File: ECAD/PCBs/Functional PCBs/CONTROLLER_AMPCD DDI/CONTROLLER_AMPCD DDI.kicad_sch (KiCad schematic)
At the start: 49 parts, among them IC1 THVD1410DR, IC2 TPS563300DRLR, J1 BUS IN, J2 BUS OUT, J3 DDI/AMPCD, J4 BRT/CRS, J5 CONT/HDG, J6 DDI ROT, J7 AMPCD ROT, J8 EWI SW, Q1 AO3400A, Q2 IRLML6402TRPBF

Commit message: Updating Symbols to new/corrected library entries
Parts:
- C2: symbol Device:C -> OH_Symbols:Capacitor_0603_10uF
- C3: symbol Device:C -> OH_Symbols:Capacitor_0402_0.1uF
- D2: LCSC (none) -> C404012
- IC1: LCSC (none) -> C2671345
- Q1: LCSC (none) -> C20917; Manufacture PN (none) -> AO3400A
- R1: symbol Device:R -> OH_Symbols:Resistor_0603_100Ω; LCSC C25804 -> C22775; PN 0603WAF1002T5E -> 0603WAF1000T5E
- R13: symbol Device:R -> OH_Symbols:Resistor_0402_0Ω; LCSC (none) -> C17168; Manufacture PN (none) -> 0402WGF0000TCE
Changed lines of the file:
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@@
 	)
 	(symbol
-		(lib_id "Device:R")
+		(lib_id "OH_Symbols:Resistor_0603_100Ω")
 		(at 33.02 177.8 270)
 		(mirror x)
@@
 			)
 		)
-		(property "Datasheet" "https://datasheet.lcsc.com/szlcsc/1811062009_UNI-ROYAL-Uniroyal-Elec-0603WAF1002T5E_C25804.pdf"
+		(property "Datasheet" "https://www.lcsc.com/datasheet/C22775.pdf"
 			(at 33.02 177.8 0)
 			(hide yes)
@@
 			)
 		)
-		(property "Description" ""
+		(property "Description" "Resistor,, SMD 0603_1608, 100 Ohm"
 			(at 33.02 177.8 0)
+			(hide yes)
 			(show_name no)
 			(do_not_autoplace no)
@@
 			)
 		)
-		(property "PN" "0603WAF1002T5E"
+		(property "PN" "0603WAF1000T5E"
 			(at 33.02 177.8 90)
 			(hide yes)
@@
 			)
 		)
-		(property "LCSC" "C25804"
+		(property "LCSC" "C22775"
 			(at 33.02 177.8 90)
 			(hide yes)
@@
 			)
 		)
+		(property "LCSC" "C20917"
+			(at 44.45 177.8 0)
+			(hide yes)
+			(show_name no)
+			(do_not_autoplace no)
+			(effects
+				(font
+					(size 1.27 1.27)
+				)
+			)
+		)
+		(property "Manufacture PN" "AO3400A"
+			(at 44.45 177.8 0)
+			(hide yes)
+			(show_name no)
+			(do_not_autoplace no)
+			(effects
+				(font
+					(size 1.27 1.27)
+				)
+			)
+		)
 		(pin "1"
 		)
@@
 			)
 		)
+		(property "LCSC" "C2671345"
+			(at 205.74 123.19 0)
+			(hide yes)
+			(show_name no)
+			(do_not_autoplace no)
+			(effects
+				(font
+					(size 1.27 1.27)
+				)
+			)
+		)
 		(pin "8"
 		)
@@
 	)
 	(symbol
-		(lib_id "Device:C")
+		(lib_id "OH_Symbols:Capacitor_0402_0.1uF")
 		(at 67.31 115.57 180)
 		(unit 1)
@@
 			)
 		)
-		(property "Description" ""
+		(property "Description" "Capacitor, Non-polarized, SMD 0402_1005, 0.1uF"
 			(at 70.231 117.9943 0)
+			(hide yes)
 			(show_name no)
 			(do_not_autoplace no)
@@
 	)
 	(symbol
-		(lib_id "Device:R")
+		(lib_id "OH_Symbols:Resistor_0402_0Ω")
 		(at 106.68 104.14 90)
 		(unit 1)
@@
 			)
 		)
-		(property "Datasheet" ""
+		(property "Datasheet" "https://www.lcsc.com/datasheet/C17168.pdf"
+			(at 106.68 104.14 0)
+			(hide yes)
+			(show_name no)
+			(do_not_autoplace no)
+			(effects
+				(font
+					(size 1.27 1.27)
+				)
+			)
+		)
+		(property "Description" "Resistor,, SMD 0402_1005, 0 Ohm"
+			(at 106.68 104.14 0)
+			(hide yes)
+			(show_name no)
+			(do_not_autoplace no)
+			(effects
+				(font
+					(size 1.27 1.27)
+				)
+			)
+		)
+		(property "LCSC" "C17168"
 			(at 106.68 104.14 0)
 			(hide yes)
@@
 			)
 		)
-		(property "Description" "Resistor"
+		(property "Manufacture PN" "0402WGF0000TCE"
 			(at 106.68 104.14 0)
 			(hide yes)
@@
 	)
 	(symbol
-		(lib_id "Device:C")
+		(lib_id "OH_Symbols:Capacitor_0603_10uF")
 		(at 60.96 115.57 0)
 		(mirror x)
@@
 			)
 		)
-		(property "Description" ""
+		(property "Description" "Capacitor, Non-polarized, SMD 0603_1608, 10uF"
 			(at 58.039 117.9943 0)
+			(hide yes)
 			(show_name no)
 			(do_not_autoplace no)
@@
 			)
 		)
+		(property "LCSC" "C404012"
+			(at 246.38 127 0)
+			(hide yes)
+			(show_name no)
+			(do_not_autoplace no)
+			(effects
+				(font
+					(size 1.27 1.27)
+				)
+			)
+		)

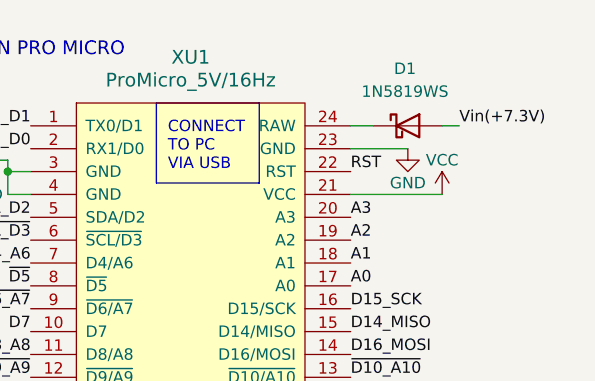
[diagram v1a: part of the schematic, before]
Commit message: Created MCAD and ECAD Release
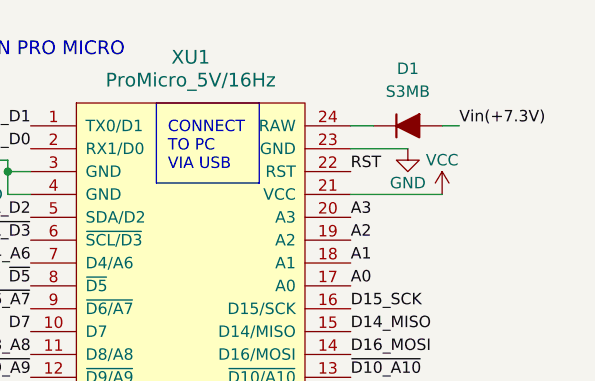
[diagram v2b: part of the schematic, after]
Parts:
- removed D1: 1N5819WS, Diode_SMD:D_SOD-323_HandSoldering, symbol OH_Symbols:1N5819WS
- added D1: S3MB, Diode_SMD:D_SMB, symbol OH_Symbols:D_Filled
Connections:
- net Vin(+7.3V): now also D1.2 (A)
- net at XU1.24 (RAW): now also D1.1 (K)
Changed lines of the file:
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@@
+	)
+	(symbol
+		(lib_id "OH_Symbols:D_Filled")
+		(at 251.46 24.13 0)
+		(unit 1)
+		(body_style 1)
+		(exclude_from_sim no)
+		(in_bom yes)
+		(on_board yes)
+		(in_pos_files yes)
+		(dnp no)
+		(fields_autoplaced yes)
+		(property "Reference" "D1"
+			(at 251.46 17.78 0)
+			(show_name no)
+			(do_not_autoplace no)
+			(effects
+				(font
+					(size 1.27 1.27)
+				)
+			)
+		)
+		(property "Value" "S3MB"
+			(at 251.46 20.32 0)
+			(show_name no)
+			(do_not_autoplace no)
+			(effects
+				(font
+					(size 1.27 1.27)
+				)
+			)
+		)
+		(property "Footprint" "Diode_SMD:D_SMB"
+			(at 264.16 117.78 0)
+			(hide yes)
+			(show_name no)
+			(do_not_autoplace no)
+			(effects
+				(font
+					(size 1.27 1.27)
+				)
+				(justify left top)
+			)
+		)
+		(property "Datasheet" "https://www.lcsc.com/datasheet/C47524.pdf?spm=wm.sxq.inf.ggs&lcsc_vid=QgMIUFNeEwUNV1dQFVgIUVVXFlcNBV1eEgJfVldQFgcxVlNeTlJdU11SR1NYUDsOAxUeFF5JWBYZEEoKFBINSQcJGk4%3D"
+			(at 251.46 24.13 0)
+			(hide yes)
+			(show_name no)
+			(do_not_autoplace no)
+			(effects
+				(font
+					(size 1.27 1.27)
+				)
+			)
+		)
+		(property "Description" "3 A, 1000 V"
+			(at 251.46 24.13 0)
+			(hide yes)
+			(show_name no)
+			(do_not_autoplace no)
+			(effects
+				(font
+					(size 1.27 1.27)
+				)
+			)
+		)
+		(property "LCSC" "C47524"
+			(at 251.46 24.13 0)
+			(hide yes)
+			(show_name no)
+			(do_not_autoplace no)
+			(effects
+				(font
+					(size 1.27 1.27)
+				)
+			)
+		)
+		(property "Manufacturer PN" "S3MB"
+			(at 251.46 24.13 0)
+			(hide yes)
+			(show_name no)
+			(do_not_autoplace no)
+			(effects
+				(font
+					(size 1.27 1.27)
+				)
+			)
+		)
+		(property "Manufacturer_Name" "MDD(Microdiode Semiconductor)"
+			(at 264.16 517.78 0)
+			(hide yes)
+			(show_name no)
+			(do_not_autoplace no)
+			(effects
+				(font
+					(size 1.27 1.27)
+				)
+				(justify left top)
+			)
+		)
+		(property "Arrow Part Number" ""
+			(at 251.46 24.13 0)
+			(hide yes)
+			(show_name no)
+			(do_not_autoplace no)
+			(effects
+				(font
+					(size 1.27 1.27)
+				)
+			)
+		)
+		(property "Arrow Price/Stock" ""
+			(at 251.46 24.13 0)
+			(hide yes)
+			(show_name no)
+			(do_not_autoplace no)
+			(effects
+				(font
+					(size 1.27 1.27)
+				)
+			)
+		)
+		(property "Height" ""
+			(at 251.46 24.13 0)
+			(hide yes)
+			(show_name no)
+			(do_not_autoplace no)
+			(effects
+				(font
+					(size 1.27 1.27)
+				)
+			)
+		)
+		(property "Manufacturer_Part_Number" ""
+			(at 251.46 24.13 0)
+			(hide yes)
+			(show_name no)
+			(do_not_autoplace no)
+			(effects
+				(font
+					(size 1.27 1.27)
+				)
+			)
+		)
+		(property "Mouser Part Number" ""
+			(at 251.46 24.13 0)
+			(hide yes)
+			(show_name no)
+			(do_not_autoplace no)
+			(effects
+				(font
+					(size 1.27 1.27)
+				)
+			)
+		)
+		(property "Mouser Price/Stock" ""
+			(at 251.46 24.13 0)
+			(hide yes)
+			(show_name no)
+			(do_not_autoplace no)
+			(effects
+				(font
+					(size 1.27 1.27)
+				)
+			)
+		)
+		(property "Sim.Device" "D"
+			(at 251.46 24.13 0)
+			(hide yes)
+			(show_name no)
+			(do_not_autoplace no)
+			(effects
+				(font
+					(size 1.27 1.27)
+				)
+			)
+		)
+		(property "Sim.Pins" "1=K 2=A"
+			(at 251.46 24.13 0)
+			(hide yes)
+			(show_name no)
+			(do_not_autoplace no)
+			(effects
+				(font
+					(size 1.27 1.27)
+				)
+			)
+		)
+		(pin "1"
+		)
+		(pin "2"
+		)
+		(instances
+			(project "CONTROLLER_AMPCD DDI"
+				(path "/90801baf-c3c5-4643-9dee-a3d06555aba9"
+					(reference "D1")
+					(unit 1)
+				)
+			)
+		)
 	)
 	(symbol
@@
 					(unit 1)
 				)
-			)
-		)
-	)
-	(symbol
-		(lib_id "OH_Symbols:1N5819WS")
-		(at 251.46 24.13 0)
-		(unit 1)
-		(body_style 1)
-		(exclude_from_sim no)
-		(in_bom yes)
-		(on_board yes)
-		(in_pos_files yes)
-		(dnp no)
-		(fields_autoplaced yes)
-		(property "Reference" "D1"
-			(at 251.1425 17.78 0)
-			(show_name no)
-			(do_not_autoplace no)
-			(effects
-				(font
-					(size 1.27 1.27)
-				)
-			)
-		)
-		(property "Value" "1N5819WS"
-			(at 251.1425 20.32 0)
-			(show_name no)
-			(do_not_autoplace no)
-			(effects
-				(font
-					(size 1.27 1.27)
-				)
-			)
-		)
-		(property "Footprint" "Diode_SMD:D_SOD-323_HandSoldering"
-			(at 251.46 24.13 0)
-			(hide yes)
-			(show_name no)
-			(do_not_autoplace no)
-			(effects
-				(font
-					(size 1.27 1.27)
-				)
-			)
-		)
-		(property "Datasheet" "https://datasheet.lcsc.com/lcsc/2204281430_Guangdong-Hottech-1N5819WS_C191023.pdf"
-			(at 251.46 24.13 0)
-			(hide yes)
-			(show_name no)
-			(do_not_autoplace no)
-			(effects
-				(font
-					(size 1.27 1.27)
-				)
-			)
-		)
-		(property "Description" ""
-			(at 251.46 24.13 0)
-			(show_name no)
-			(do_not_autoplace no)
-			(effects
-				(font
-					(size 1.27 1.27)
-				)
-			)
-		)
-		(property "LCSC" "C191023"
-			(at 251.46 24.13 0)
-			(hide yes)
-			(show_name no)
-			(do_not_autoplace no)
-			(effects
-				(font
-					(size 1.27 1.27)
-				)
-			)
-		)
-		(property "Manufacturer PN" "1N5819WS"
-			(at 251.46 24.13 0)
-			(hide yes)
-			(show_name no)
-			(do_not_autoplace no)
-			(effects
-				(font
-					(size 1.27 1.27)
-				)
-			)
-		)
-		(pin "1"
-		)
-		(pin "2"
-		)
-		(instances
-			(project "ABSIS_ALE"
-				(path "/033779dd-769d-40f0-a337-a3f830befbfb"
-					(reference "D1")
-					(unit 1)
-				)
-			)
-			(project "CONTROLLER_AMPCD DDI"
-				(path "/90801baf-c3c5-4643-9dee-a3d06555aba9"
-					(reference "D1")
-					(unit 1)
-				)
